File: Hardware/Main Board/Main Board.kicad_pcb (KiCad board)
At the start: 2 copper layers, 59 parts, among them J1 Micro_SD_Card_Det1, J2 Camera Module, J3 Conn_01x09_Socket, J4 MIC 1 Connector, J5 MIC 2 Connector, J6 USB_C_Receptacle_USB2.0_16P, J7 OLED, U1 ESP32-S3-WROOM-2, U2 TPS63060, U3 TP4056-42-ESOP8

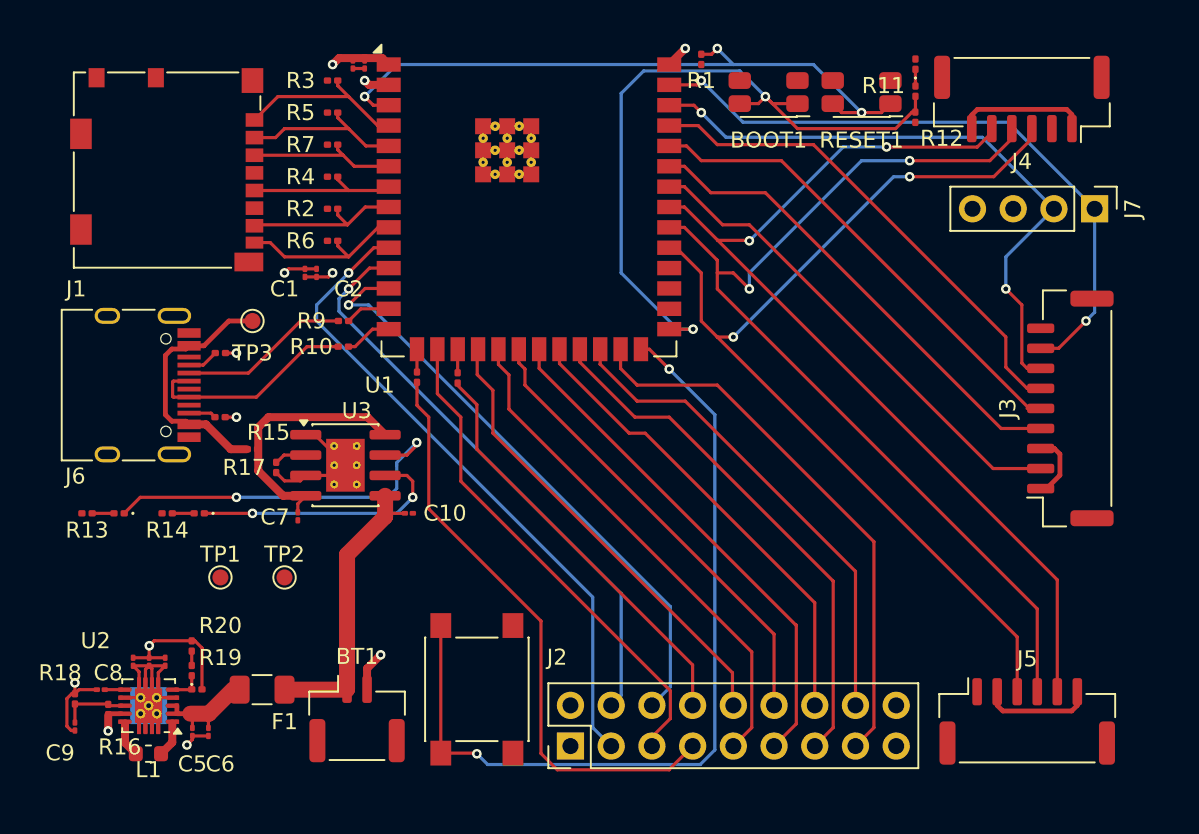
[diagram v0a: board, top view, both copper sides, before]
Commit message: reviewed most of main board, getting ready to finalize and prepare for manufacturing
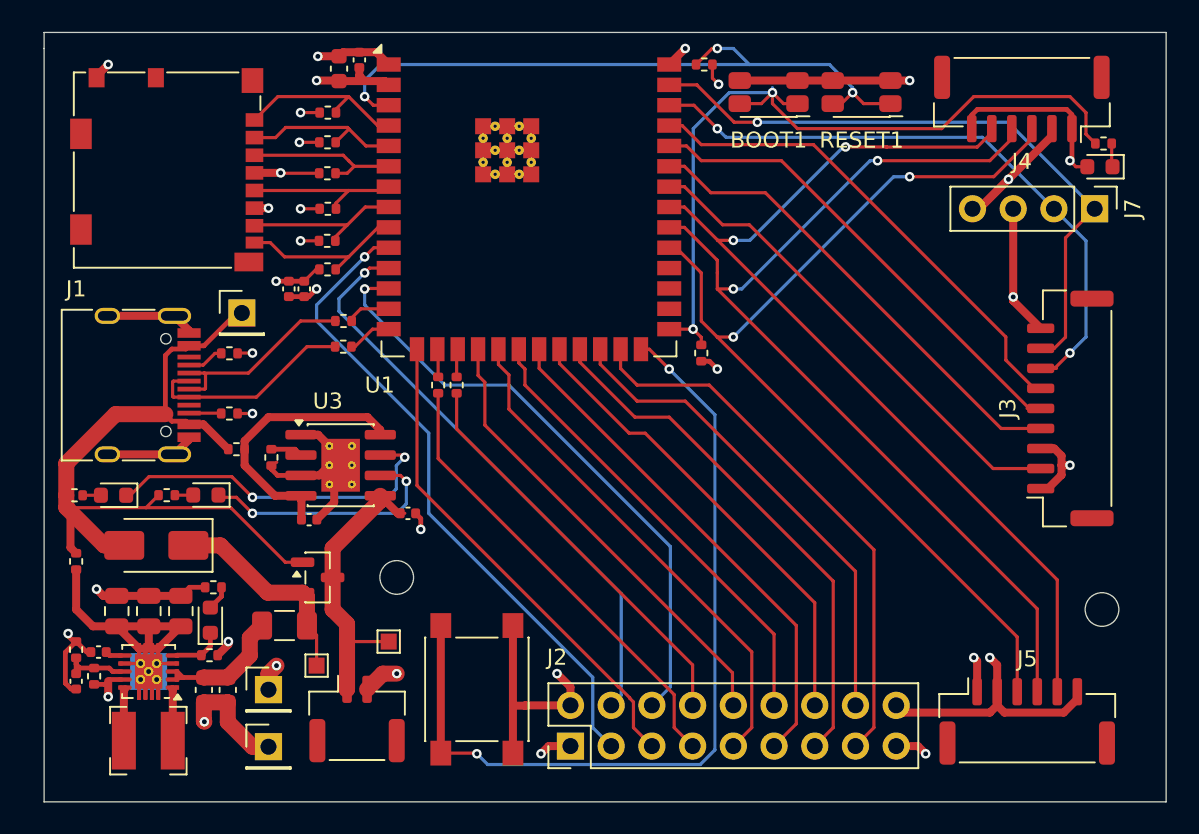
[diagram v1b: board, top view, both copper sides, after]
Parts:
- added D5: SS14, Diode_SMD:D_SMA, F.Cu at (81.0, 80.0)
- added H1: MountingHole, MountingHole:MountingHole_2.1mm, F.Cu at (96.0, 82.0)
- added H2: MountingHole, MountingHole:MountingHole_2.1mm, F.Cu at (140.0, 84.0)
- added Q1: AO3401A, Package_TO_SOT_SMD:SOT-23, F.Cu at (91.1, 82.0)
- added R24: 100k, Resistor_SMD:R_0402_1005Metric, F.Cu at (76.0, 81.0)
- added TP4: TestPoint, TestPoint:TestPoint_Pad_1.0x1.0mm, F.Cu at (91.0, 87.5)
- added TP5: TestPoint, TestPoint:TestPoint_Pad_1.0x1.0mm, F.Cu at (95.5, 86.0)
- C1, C10, C2, C3, C7, C8, C9: footprint Capacitor_SMD:C_01005_0402Metric -> Capacitor_SMD:C_0402_1005Metric
- C11, C12, C13: footprint Capacitor_SMD:C_01005_0402Metric -> Capacitor_SMD:C_0805_2012Metric
- C4, C5, C6: footprint Capacitor_SMD:C_01005_0402Metric -> Capacitor_SMD:C_0603_1608Metric
- D1, D2, D3, D4: footprint LED_SMD:LED_0201_0603Metric -> LED_SMD:LED_0603_1608Metric
- L1: footprint Inductor_SMD:L_0603_1608Metric -> Inductor_SMD:L_Bourns-SRN4018
- R1, R10, R11, R12, R13, R14, R15, R16, R17, R18, R19, R2, R20, R21, R22, R23, R3, R4, R5, R6, R7, R8, R9: footprint Resistor_SMD:R_0201_0603Metric -> Resistor_SMD:R_0402_1005Metric
- TP1, TP2, TP3: footprint TestPoint:TestPoint_Pad_D1.0mm -> Connector_PinHeader_2.54mm:PinHeader_1x01_P2.54mm_Vertical
- moved R12 19.9 mm to (115.0, 68.0)
- moved D1 13.2 mm to (139.9, 56.4), turned to 180 degrees
- moved R11 12.2 mm to (140.1, 54.9), turned to 0 degrees
- moved TP1 11.0 mm to (88.0, 92.6)
- moved TP2 7.07 mm to (88.0, 89.0)
- moved C12 4.37 mm to (78.5, 84.1)
- moved C11 4.34 mm to (82.5, 84.1)
- moved F1 4.24 mm to (89.0, 85.0)
- moved R20 3.90 mm to (84.6, 82.6), turned to 180 degrees
- moved D4 3.35 mm to (84.4, 84.7)
- moved C13 3.16 mm to (80.5, 84.1)
- moved R18 3.07 mm to (76.0, 86.5)
- moved C6 2.89 mm to (85.5, 89.0)
- moved C9 2.82 mm to (76.0, 88.5)
- moved C5 2.72 mm to (84.0, 89.0)
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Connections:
- F1 pad 1: +BATT -> VIN
- R8 pad 1: Net-(U1-IO3) -> Net-(U1-IO46)
- U1 pad 15: Net-(U1-IO3) -> CAM_VSYNC
- U1 pad 16: CAM_VSYNC -> Net-(U1-IO46)
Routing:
- net GND: track 47.0 -> 124.0 mm, vias 8 -> 16
- net +3.3V: track 23.4 -> 59.0 mm, vias 4 -> 18
- net +5V_USB: track 16.1 -> 49.3 mm
- net VIN: track 0.00 -> 13.3 mm
- net CAM_PCLK: track 36.9 -> 28.6 mm
- net Net-(U1-IO0): track 44.4 -> 49.9 mm
- net USB_D-: track 10.7 -> 12.7 mm
- net Net-(U2-EN): track 6.51 -> 8.38 mm
- net Net-(U1-IO46): track 0.00 -> 1.83 mm
- net Net-(D2-K): track 23.4 -> 21.9 mm
- net Net-(U1-IO3): track 1.43 -> 0.00 mm
- net Net-(U1-EN): track 41.4 -> 42.8 mm
- net Net-(D4-K): track 1.83 -> 3.19 mm
- net Net-(U2-L2): track 2.18 -> 3.25 mm
- net Net-(U2-L1): track 2.20 -> 3.23 mm
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- added copper zone on In2.Cu, net +3.3V
- added copper zone on In1.Cu, net GND
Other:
- board outline added: 70 x 48 mm
- copper layers 2 -> 4
- board text removed: "${REFERENCE}"
